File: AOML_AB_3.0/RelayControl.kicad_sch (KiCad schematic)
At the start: 38 parts, among them IC1 CD4043BDR, IC2 CD4043BDR, J5 Conn_01x03, K1 TX2-L2-5V, K10 TX2-L2-5V, K11 TX2-L2-5V, K13 TX2-L2-5V, K2 TX2-L2-5V, K3 TX2-L2-5V, K4 TX2-L2-5V, K5 TX2-L2-5V, K6 TX2-L2-5V, K7 TX2-L2-5V, K8 TX2-L2-5V, K9 TX2-L2-5V, U10 TLP170AM, U11 TLP170AM, U12 TLP170AM, U13 TLP170AM, U14 TLP170AM, U15 TLP170AM, U16 TLP170AM, U17 TLP170AM, U5 ULN2003ADR

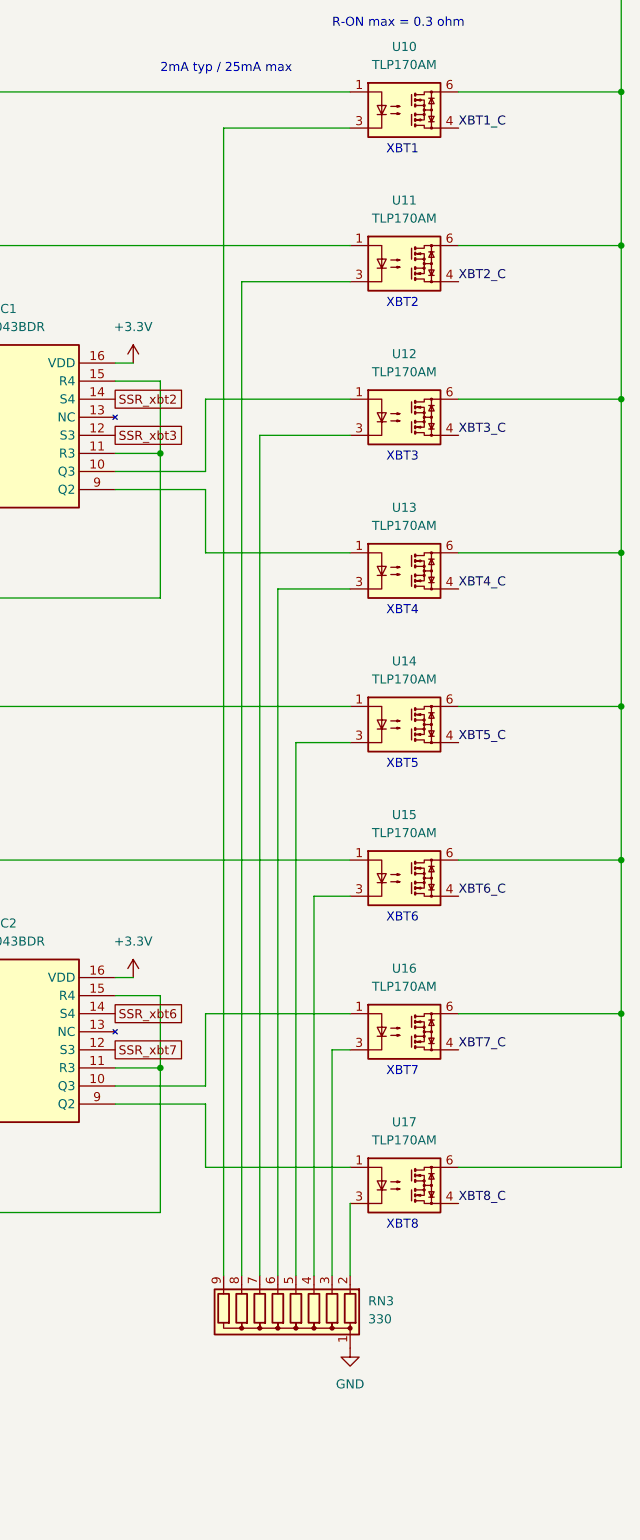
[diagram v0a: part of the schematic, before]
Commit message: PCB layout finished, next step is routing
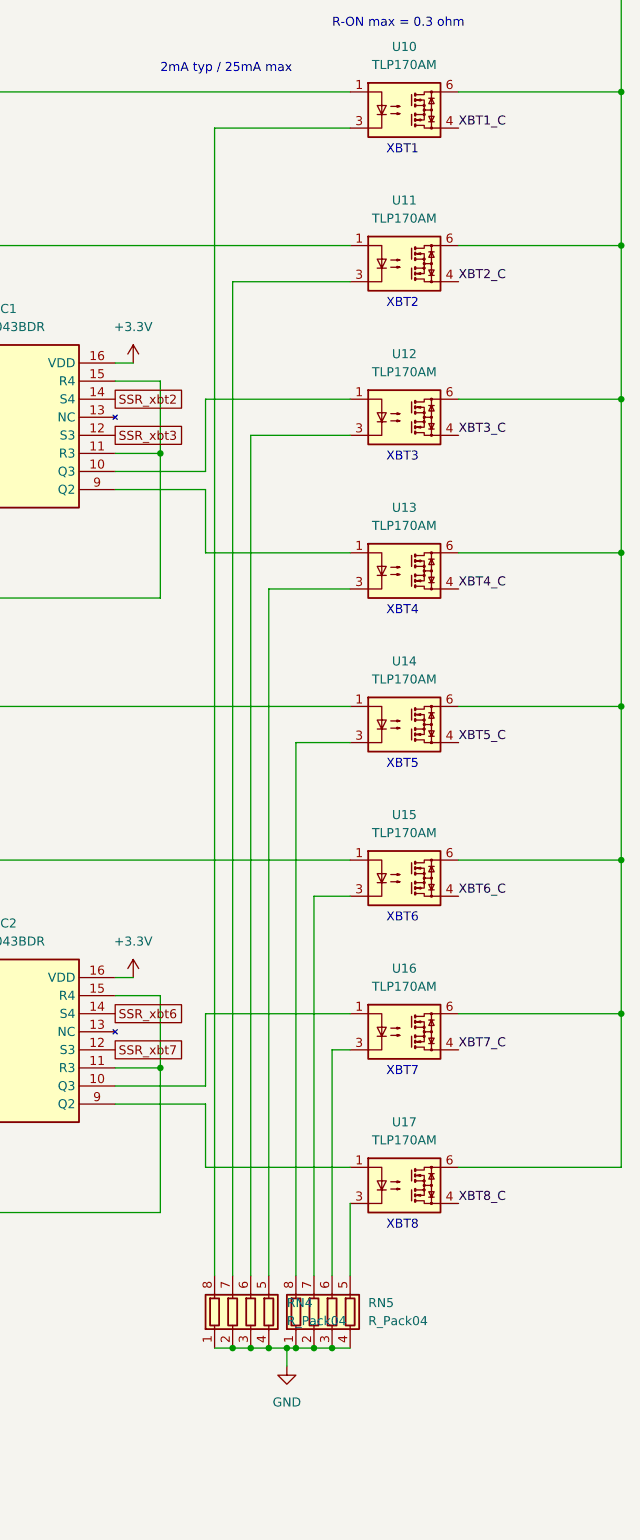
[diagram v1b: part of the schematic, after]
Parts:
- removed RN3: 330, Resistor_network-330:RESCAV80P400X210X65-10N, symbol Device:R_Network08
- added RN4, RN5: R_Pack04, Resistor_network_x4_-330:RESCAXE80P320X160X70-8N, symbol Device:R_Pack04
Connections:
- net GND: now also RN4.1 (R1.1), RN4.2 (R2.1), RN4.3 (R3.1), RN4.4 (R4.1), RN5.1 (R1.1), RN5.2 (R2.1), RN5.3 (R3.1), RN5.4 (R4.1)
- net at U14.3: now also RN5.8 (R1.2)
- net at U12.3: now also RN4.6 (R3.2)
- net at U13.3: now also RN4.5 (R4.2)
- net at U15.3: now also RN5.7 (R2.2)
- net at U17.3: now also RN5.5 (R4.2)
- net at U16.3: now also RN5.6 (R3.2)
- net at U11.3: now also RN4.7 (R2.2)
- net at U10.3: now also RN4.8 (R1.2)
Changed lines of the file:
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@@
   (junction (at 331.47 110.49) (diameter 0) (color 0 0 0 0)
   )
+  (junction (at 341.63 236.22) (diameter 0) (color 0 0 0 0)
+  )
   (junction (at 138.43 110.49) (diameter 0) (color 0 0 0 0)
   )
@@
   (junction (at 396.24 189.23) (diameter 0) (color 0 0 0 0)
   )
+  (junction (at 344.17 236.22) (diameter 0) (color 0 0 0 0)
+  )
   (junction (at 138.43 137.16) (diameter 0) (color 0 0 0 0)
   )
@@
   (junction (at 220.98 196.85) (diameter 0) (color 0 0 0 0)
   )
+  (junction (at 355.6 236.22) (diameter 0) (color 0 0 0 0)
+  )
   (junction (at 143.51 223.52) (diameter 0) (color 0 0 0 0)
   )
@@
   (junction (at 143.51 153.67) (diameter 0) (color 0 0 0 0)
   )
+  (junction (at 353.06 236.22) (diameter 0) (color 0 0 0 0)
+  )
   (junction (at 193.04 142.24) (diameter 0) (color 0 0 0 0)
   )
@@
   (junction (at 396.24 167.64) (diameter 0) (color 0 0 0 0)
   )
+  (junction (at 346.71 236.22) (diameter 0) (color 0 0 0 0)
+  )
   (junction (at 198.12 153.67) (diameter 0) (color 0 0 0 0)
   )
   (junction (at 151.13 241.3) (diameter 0) (color 0 0 0 0)
   )
+  (junction (at 349.25 236.22) (diameter 0) (color 0 0 0 0)
+  )
+  (junction (at 350.52 236.22) (diameter 0) (color 0 0 0 0)
+  )
   (junction (at 151.13 228.6) (diameter 0) (color 0 0 0 0)
   )
@@
     (stroke (width 0) (type default))
   )
-  (wire (pts (xy 345.44 226.06) (xy 345.44 107.95))
+  (wire (pts (xy 344.17 226.06) (xy 344.17 107.95))
     (stroke (width 0) (type default))
   )
@@
     (stroke (width 0) (type default))
   )
-  (wire (pts (xy 340.36 226.06) (xy 340.36 64.77))
+  (wire (pts (xy 339.09 226.06) (xy 339.09 64.77))
     (stroke (width 0) (type default))
   )
@@
     (stroke (width 0) (type default))
   )
+  (wire (pts (xy 344.17 236.22) (xy 346.71 236.22))
+    (stroke (width 0) (type default))
+  )
   (wire (pts (xy 77.47 173.99) (xy 157.48 173.99))
     (stroke (width 0) (type default))
@@
     (stroke (width 0) (type default))
   )
-  (wire (pts (xy 345.44 107.95) (xy 358.14 107.95))
+  (wire (pts (xy 344.17 107.95) (xy 358.14 107.95))
     (stroke (width 0) (type default))
   )
@@
     (stroke (width 0) (type default))
   )
-  (wire (pts (xy 347.98 226.06) (xy 347.98 129.54))
+  (wire (pts (xy 346.71 226.06) (xy 346.71 129.54))
     (stroke (width 0) (type default))
   )
@@
     (stroke (width 0) (type default))
   )
-  (wire (pts (xy 340.36 64.77) (xy 358.14 64.77))
+  (wire (pts (xy 339.09 64.77) (xy 358.14 64.77))
     (stroke (width 0) (type default))
   )
@@
     (stroke (width 0) (type default))
   )
+  (wire (pts (xy 341.63 236.22) (xy 344.17 236.22))
+    (stroke (width 0) (type default))
+  )
   (wire (pts (xy 133.35 194.31) (xy 144.78 194.31))
     (stroke (width 0) (type default))
@@
     (stroke (width 0) (type default))
   )
-  (wire (pts (xy 342.9 226.06) (xy 342.9 86.36))
+  (wire (pts (xy 341.63 226.06) (xy 341.63 86.36))
     (stroke (width 0) (type default))
   )
@@
     (stroke (width 0) (type default))
   )
+  (wire (pts (xy 355.6 236.22) (xy 358.14 236.22))
+    (stroke (width 0) (type default))
+  )
   (wire (pts (xy 135.89 189.23) (xy 135.89 184.15))
     (stroke (width 0) (type default))
@@
     (stroke (width 0) (type default))
   )
-  (wire (pts (xy 347.98 129.54) (xy 358.14 129.54))
+  (wire (pts (xy 346.71 129.54) (xy 358.14 129.54))
     (stroke (width 0) (type default))
   )
@@
     (stroke (width 0) (type default))
   )
+  (wire (pts (xy 353.06 236.22) (xy 355.6 236.22))
+    (stroke (width 0) (type default))
+  )
   (wire (pts (xy 198.12 153.67) (xy 203.2 153.67))
     (stroke (width 0) (type default))
@@
     (stroke (width 0) (type default))
   )
-  (wire (pts (xy 342.9 86.36) (xy 358.14 86.36))
+  (wire (pts (xy 341.63 86.36) (xy 358.14 86.36))
     (stroke (width 0) (type default))
   )
@@
     (stroke (width 0) (type default))
   )
+  (wire (pts (xy 339.09 236.22) (xy 341.63 236.22))
+    (stroke (width 0) (type default))
+  )
   (wire (pts (xy 396.24 189.23) (xy 396.24 210.82))
     (stroke (width 0) (type default))
@@
     (stroke (width 0) (type default))
   )
+  (wire (pts (xy 346.71 236.22) (xy 349.25 236.22))
+    (stroke (width 0) (type default))
+  )
   (wire (pts (xy 396.24 102.87) (xy 373.38 102.87))
     (stroke (width 0) (type default))
@@
     (stroke (width 0) (type default))
   )
+  (wire (pts (xy 350.52 236.22) (xy 353.06 236.22))
+    (stroke (width 0) (type default))
+  )
   (wire (pts (xy 325.12 186.69) (xy 331.47 186.69))
     (stroke (width 0) (type default))
@@
     (stroke (width 0) (type default))
   )
+  (wire (pts (xy 349.25 236.22) (xy 349.25 238.76))
+    (stroke (width 0) (type default))
+  )
   (wire (pts (xy 187.96 173.99) (xy 198.12 173.99))
     (stroke (width 0) (type default))
@@
     (stroke (width 0) (type default))
   )
+  (wire (pts (xy 349.25 236.22) (xy 350.52 236.22))
+    (stroke (width 0) (type default))
+  )
   (wire (pts (xy 290.83 97.79) (xy 294.64 97.79))
     (stroke (width 0) (type default))
@@
     )
   )
-  (symbol (lib_id "power:GND") (at 358.14 236.22 0) (unit 1)
+  (symbol (lib_id "power:GND") (at 349.25 238.76 0) (unit 1)
     (in_bom yes) (on_board yes) (dnp no) (fields_autoplaced)
-    (property "Reference" "#PWR087" (at 358.14 242.57 0)
+    (property "Reference" "#PWR087" (at 349.25 245.11 0)
       (effects (font (size 1.27 1.27)) hide)
     )
-    (property "Value" "GND" (at 358.14 241.3 0)
+    (property "Value" "GND" (at 349.25 243.84 0)
       (effects (font (size 1.27 1.27)))
     )
-    (property "Footprint" "" (at 358.14 236.22 0)
+    (property "Footprint" "" (at 349.25 238.76 0)
       (effects (font (size 1.27 1.27)) hide)
     )
-    (property "Datasheet" "" (at 358.14 236.22 0)
+    (property "Datasheet" "" (at 349.25 238.76 0)
       (effects (font (size 1.27 1.27)) hide)
     )
@@
     )
   )
+  (symbol (lib_id "Device:R_Pack04") (at 355.6 231.14 0) (unit 1)
+    (in_bom yes) (on_board yes) (dnp no) (fields_autoplaced)
+    (property "Reference" "RN5" (at 360.68 229.87 0)
+      (effects (font (size 1.27 1.27)) (justify left))
+    )
+    (property "Value" "R_Pack04" (at 360.68 232.41 0)
+      (effects (font (size 1.27 1.27)) (justify left))
+    )
+    (property "Footprint" "Resistor_network_x4_-330:RESCAXE80P320X160X70-8N" (at 362.585 231.14 90)
+      (effects (font (size 1.27 1.27)) hide)
+    )
+    (property "Datasheet" "https://www.yageo.com/upload/media/product/app/datasheet/rchip/pyu-yc_tc_group_51_rohs_l.pdf" (at 355.6 231.14 0)
+      (effects (font (size 1.27 1.27)) hide)
+    )
+    (property "Digikey" "https://www.digikey.com/en/products/detail/yageo/YC164-JR-07330RL/1005112" (at 355.6 231.14 0)
+      (effects (font (size 1.27 1.27)) hide)
+    )
+    (pin "1")
+    (pin "2")
+    (pin "3")
+    (pin "4")
+    (pin "5")
+    (pin "6")
+    (pin "7")
+    (pin "8")
+    (instances
+      (project "AOML_AB_3.0"
+        (path "/6a222f58-627e-41ff-951d-9ad8d2e0d7a2/69365a30-fc6f-418a-bc31-d76af2fc83f6"
+          (reference "RN5") (unit 1)
+        )
+      )
+    )
+  )
   (symbol (lib_id "Connector_Generic:Conn_01x03") (at 248.92 148.59 180) (unit 1)
     (in_bom yes) (on_board yes) (dnp no) (fields_autoplaced)
@@
     )
   )
-  (symbol (lib_id "Device:R_Network08") (at 347.98 231.14 180) (unit 1)
-    (in_bom yes) (on_board yes) (dnp no) (fields_autoplaced)
-    (property "Reference" "RN3" (at 360.68 229.616 0)
-      (effects (font (size 1.27 1.27)) (justify right))
-    )
-    (property "Value" "330" (at 360.68 232.156 0)
-      (effects (font (size 1.27 1.27)) (justify right))
-    )
-    (property "Footprint" "Resistor_network-330:RESCAV80P400X210X65-10N" (at 335.915 231.14 90)
-      (effects (font (size 1.27 1.27)) hide)
-    )
-    (property "Datasheet" "https://industrial.panasonic.com/ww/products/pt/resistor-network-array/models/EXBE10C331J" (at 347.98 231.14 0)
-      (effects (font (size 1.27 1.27)) hide)
-    )
-    (property "Digikey" "https://www.digikey.com/en/products/detail/panasonic-electronic-components/EXB-E10C331J/282888" (at 347.98 231.14 0)
-      (effects (font (size 1.27 1.27)) hide)
-    )
-    (pin "1")
-    (pin "2")
-    (pin "3")
-    (pin "4")
-    (pin "5")
-    (pin "6")
-    (pin "7")
-    (pin "8")
-    (pin "9")
-    (instances
-      (project "AOML_AB_3.0"
-        (path "/6a222f58-627e-41ff-951d-9ad8d2e0d7a2"
-          (reference "RN3") (unit 1)
-        )
-        (path "/6a222f58-627e-41ff-951d-9ad8d2e0d7a2/69365a30-fc6f-418a-bc31-d76af2fc83f6"
-          (reference "RN4") (unit 1)
-        )
-      )
-    )
-  )
   (symbol (lib_id "Relay_SolidState:TLP175A") (at 365.76 62.23 0) (unit 1)
     (in_bom yes) (on_board yes) (dnp no) (fields_autoplaced)
@@
         )
       )
+    )
+  )
+  (symbol (lib_id "Device:R_Pack04") (at 344.17 231.14 0) (unit 1)
+    (in_bom yes) (on_board yes) (dnp no) (fields_autoplaced)
+    (property "Reference" "RN4" (at 349.25 229.87 0)
+      (effects (font (size 1.27 1.27)) (justify left))
+    )
+    (property "Value" "R_Pack04" (at 349.25 232.41 0)
+      (effects (font (size 1.27 1.27)) (justify left))
+    )
+    (property "Footprint" "Resistor_network_x4_-330:RESCAXE80P320X160X70-8N" (at 351.155 231.14 90)
+      (effects (font (size 1.27 1.27)) hide)
+    )
+    (property "Datasheet" "https://www.yageo.com/upload/media/product/app/datasheet/rchip/pyu-yc_tc_group_51_rohs_l.pdf" (at 344.17 231.14 0)
+      (effects (font (size 1.27 1.27)) hide)
+    )
+    (property "Digikey" "https://www.digikey.com/en/products/detail/yageo/YC164-JR-07330RL/1005112" (at 344.17 231.14 0)
+      (effects (font (size 1.27 1.27)) hide)
+    )
+    (pin "1")
+    (pin "2")
+    (pin "3")
+    (pin "4")
+    (pin "5")
+    (pin "6")
+    (pin "7")
+    (pin "8")
+    (instances
+      (project "AOML_AB_3.0"
+        (path "/6a222f58-627e-41ff-951d-9ad8d2e0d7a2/69365a30-fc6f-418a-bc31-d76af2fc83f6"
+          (reference "RN4") (unit 1)
+        )
+      )
